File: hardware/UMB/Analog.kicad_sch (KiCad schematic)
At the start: 54 parts, among them IC1 INA2128UA_1K, IC2 INA2128UA_1K, IC3 INA2128UA_1K, U7 TLC274AIDR, U8 TLC274AIDR, U9 TLC274AIDR

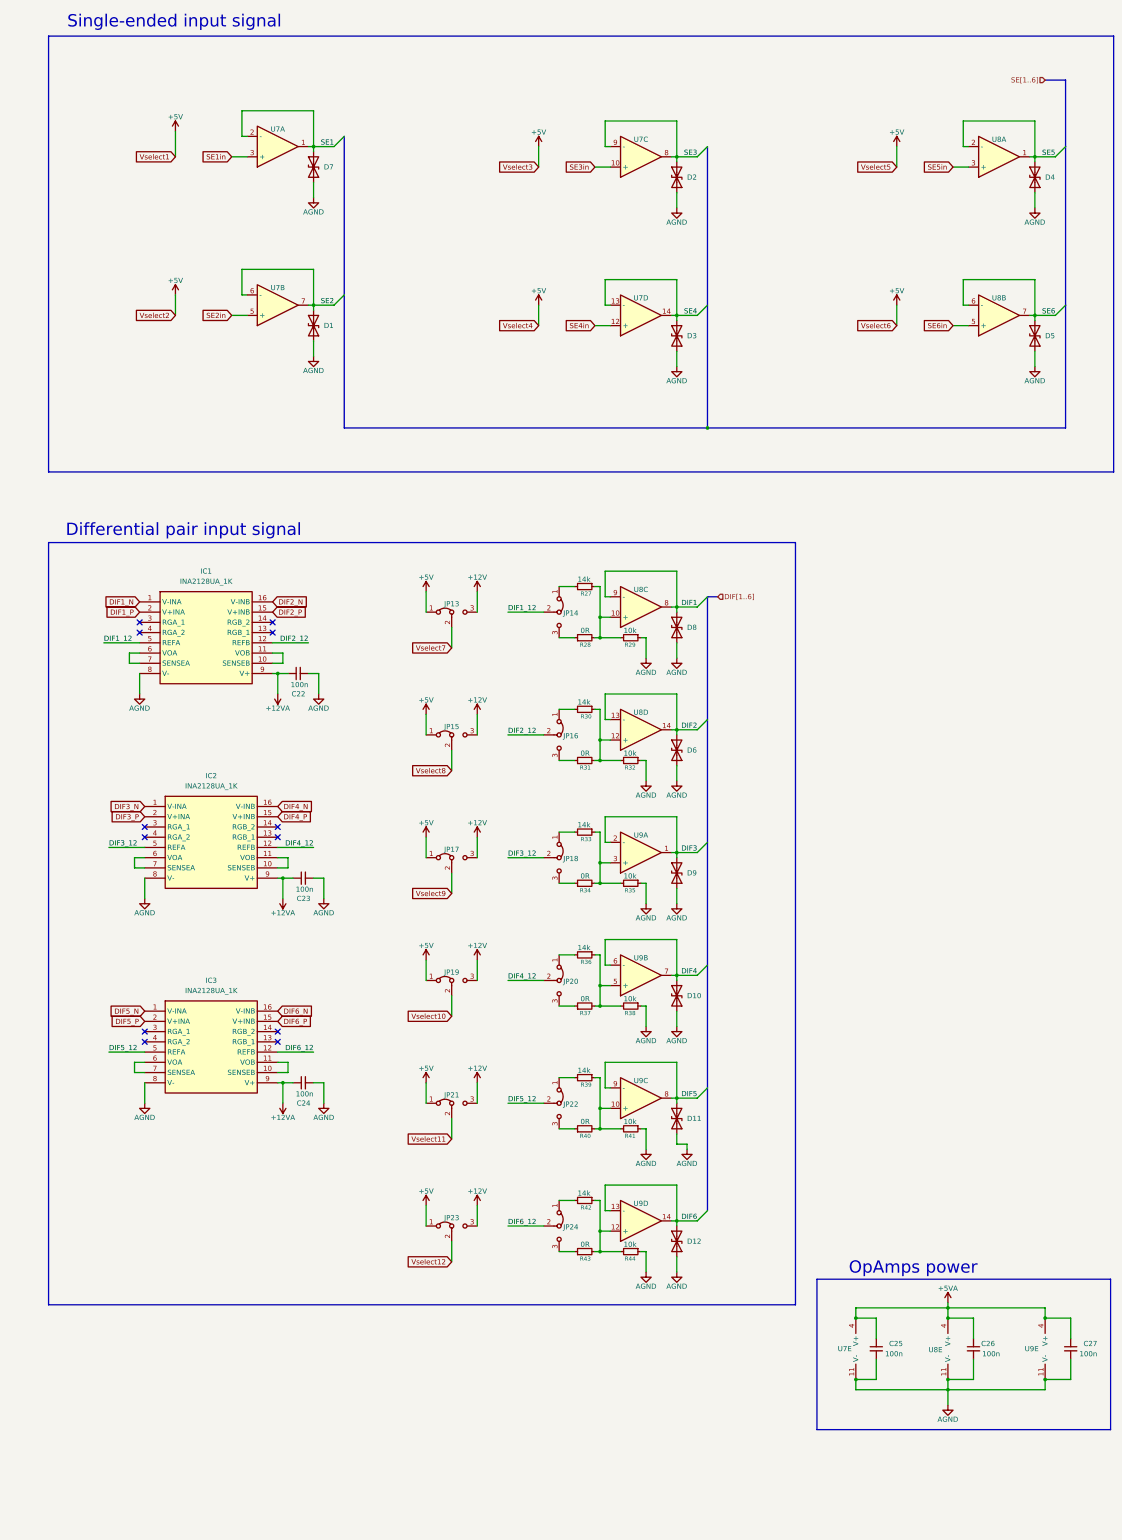
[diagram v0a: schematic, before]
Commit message: All done except power
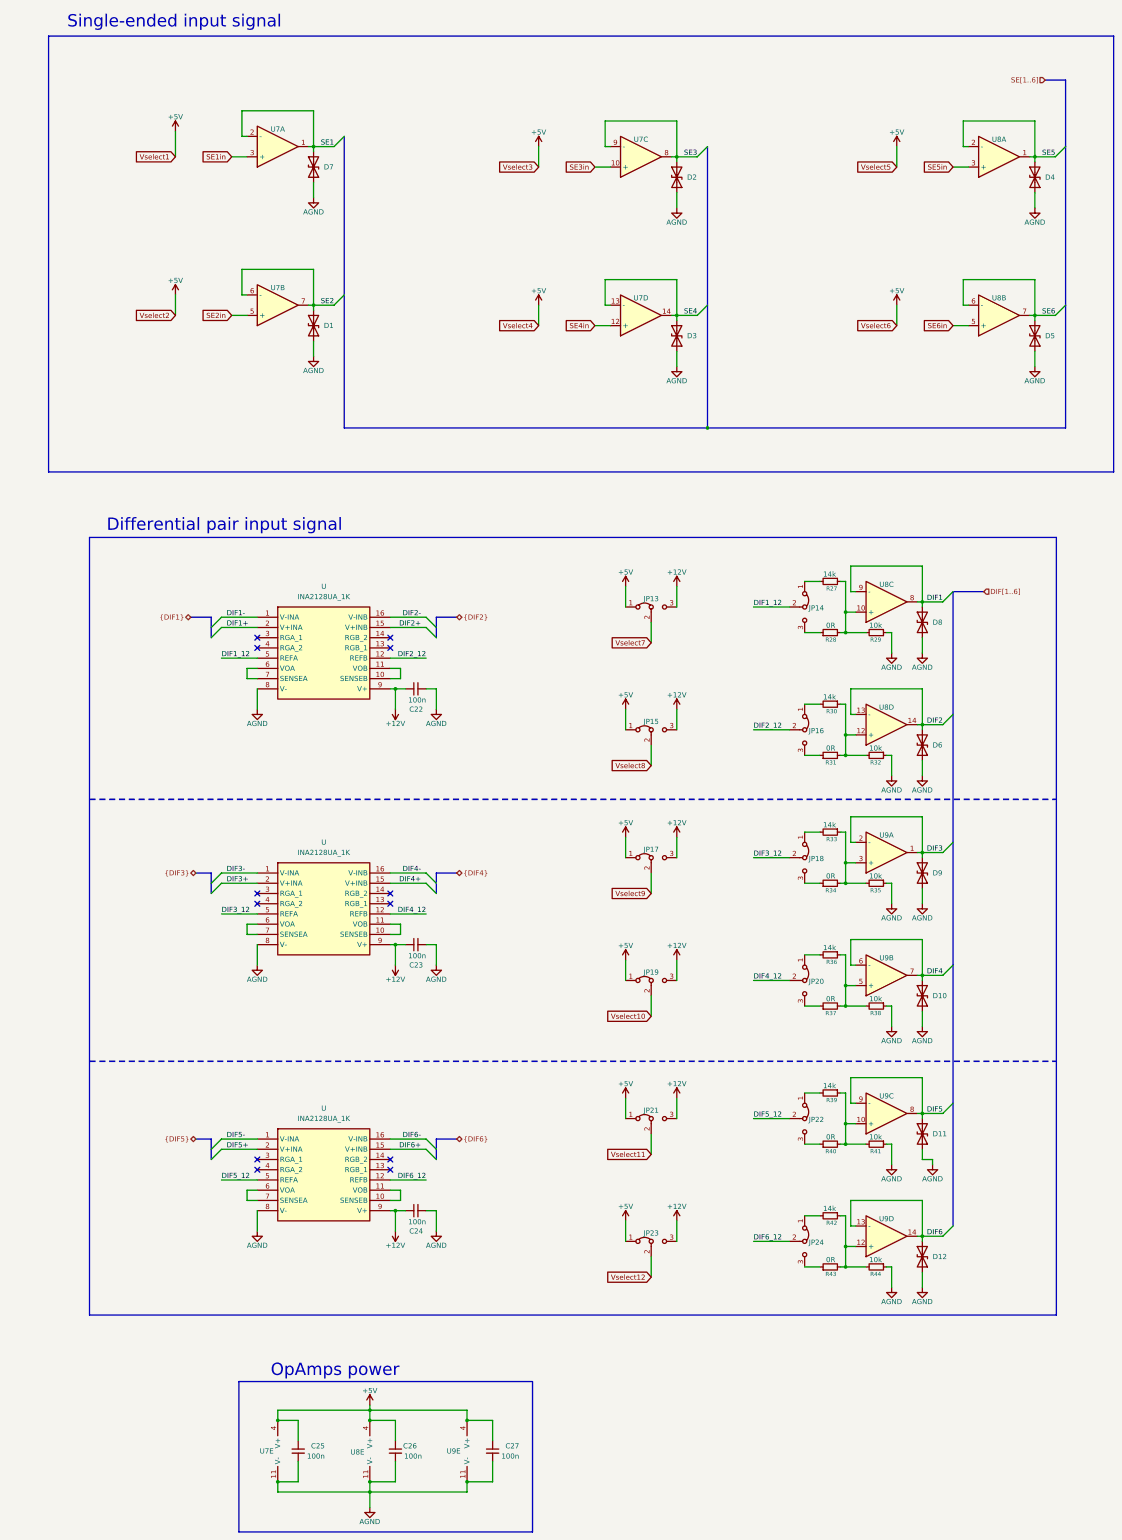
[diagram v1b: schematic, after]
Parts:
- renumbered IC3 to U, IC2 to U, IC1 to U
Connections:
- net +12VA is gone; now on net +12V: C22.1, C23.1, C24.1, U.9 (V+), U.9 (V+), U.9 (V+)
- net +5VA is gone; now on net +5V: C25.1, C26.1, C27.1, U7.4 (V+), U8.4 (V+), U9.4 (V+)
- net DIF1_N renamed DIF1-
- net DIF1_P renamed DIF1+
- net DIF2_N renamed DIF2-
- net DIF2_P renamed DIF2+
- net DIF3_N renamed DIF3-
- net DIF3_P renamed DIF3+
- net DIF4_N renamed DIF4-
- net DIF4_P renamed DIF4+
- net DIF5_N renamed DIF5-
- net DIF5_P renamed DIF5+
- net DIF6_N renamed DIF6-
- net DIF6_P renamed DIF6+
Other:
- moved on the sheet: C22, C23, C24, C25, C26, C27, D10, D11, D12, D6, D8, D9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
